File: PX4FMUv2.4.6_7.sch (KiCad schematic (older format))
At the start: 27 parts, among them J701 DF13C-2P-1.25V, U701 TCA62724FMG, U702 LT3469, U703 LRTB GFTG-T7AW-1+V7A7-29+R5T9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

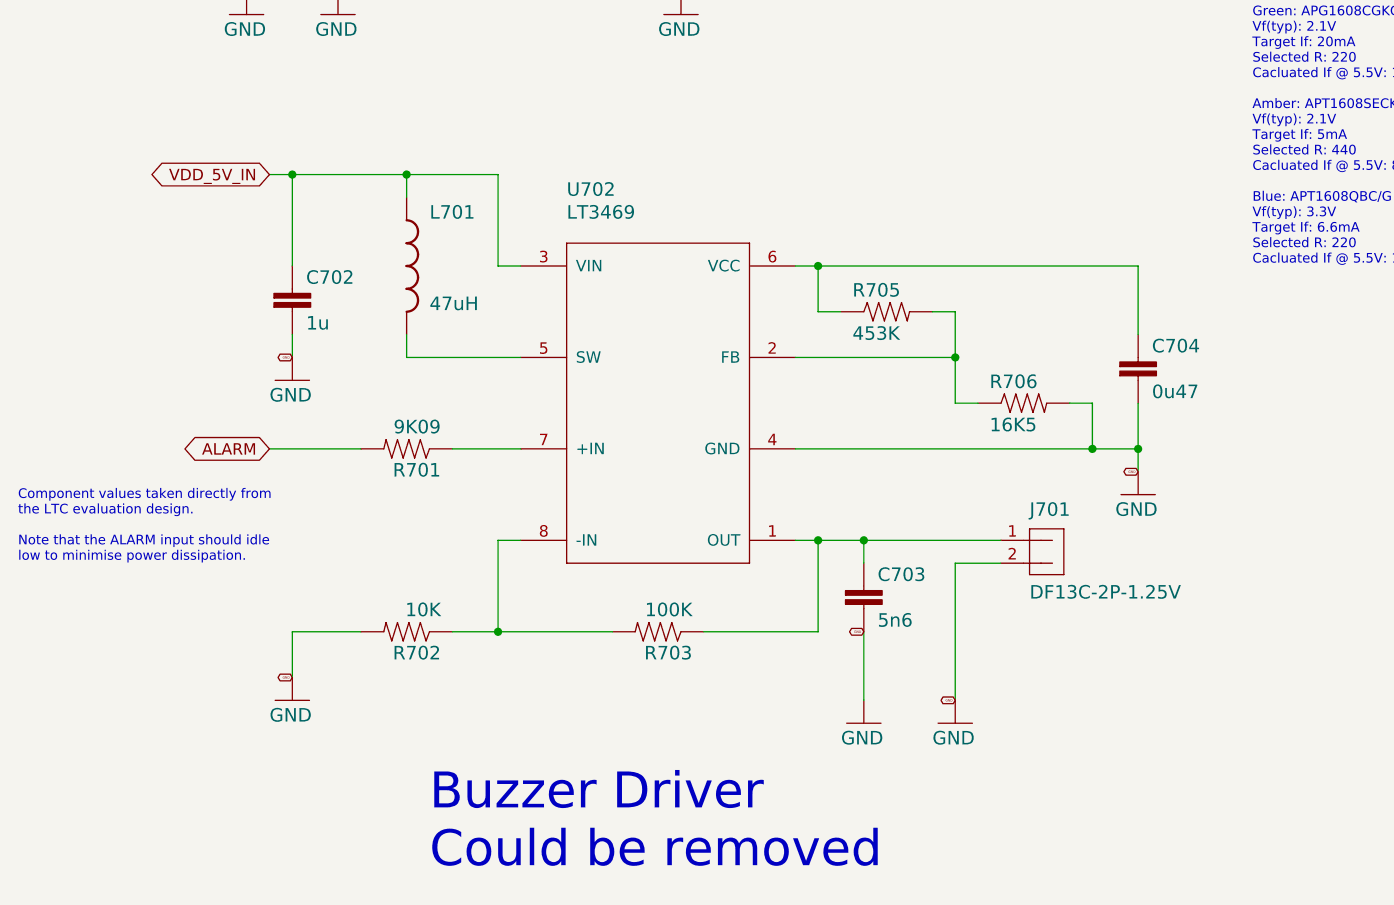
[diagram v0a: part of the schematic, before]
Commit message: removed more things
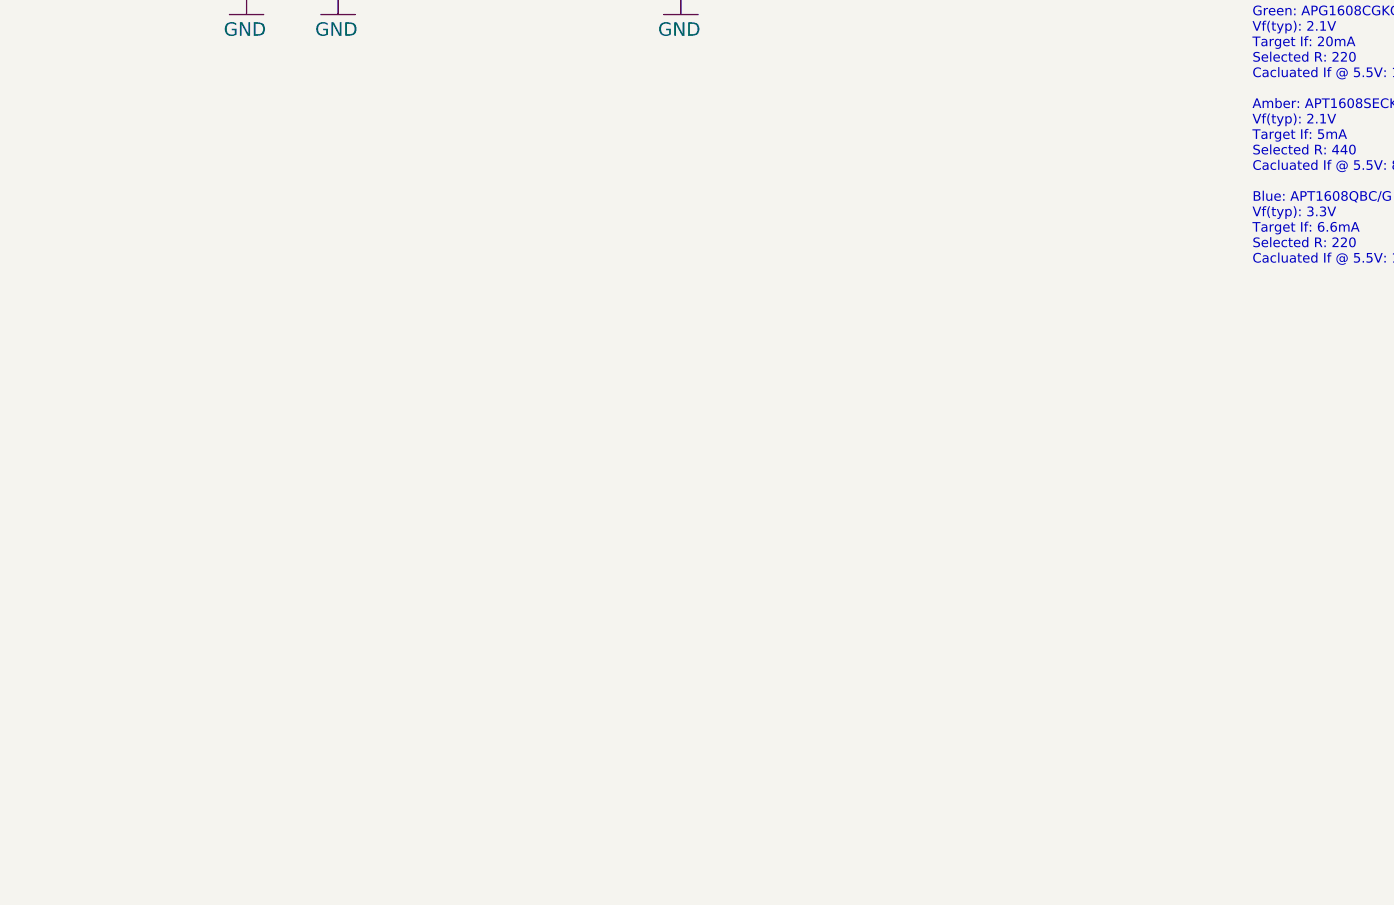
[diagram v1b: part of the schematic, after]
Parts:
- removed C702: 1u, PX4FMUv2.4.6:0603-CAP, symbol PX4FMUv2.4.6-eagle-import:CAP0603
- removed C703: 5n6, PX4FMUv2.4.6:0402-CAP, symbol PX4FMUv2.4.6-eagle-import:CAP0402
- removed C704: 0u47, PX4FMUv2.4.6:0402-CAP, symbol PX4FMUv2.4.6-eagle-import:CAP0402
- removed J701: DF13C-2P-1.25V, PX4FMUv2.4.6:DF13C-2P-1.25V, symbol PX4FMUv2.4.6-eagle-import:DF13-2P-1.25V
- removed L701: 47uH, PX4FMUv2.4.6:0805-IND, symbol PX4FMUv2.4.6-eagle-import:INDUCTOR0805
- removed R701: 9K09, PX4FMUv2.4.6:0402-RES, symbol PX4FMUv2.4.6-eagle-import:RESISTOR0402-RES
- removed R702: 10K, PX4FMUv2.4.6:0402-RES, symbol PX4FMUv2.4.6-eagle-import:RESISTOR0402-RES
- removed R703: 100K, PX4FMUv2.4.6:0402-RES, symbol PX4FMUv2.4.6-eagle-import:RESISTOR0402-RES
- removed R705: 453K, PX4FMUv2.4.6:0402-RES, symbol PX4FMUv2.4.6-eagle-import:RESISTOR0402-RES
- removed R706: 16K5, PX4FMUv2.4.6:0402-RES, symbol PX4FMUv2.4.6-eagle-import:RESISTOR0402-RES
- removed U702: LT3469, PX4FMUv2.4.6:SOT23-8, symbol PX4FMUv2.4.6-eagle-import:LT3469
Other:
- note removed: "Buzzer Driver\nCould be removed"
- note removed: "Component values taken directly from\nthe LTC evaluation design.\n\nNote that the ALARM input should idle\nlow to minimise power dissipation."
